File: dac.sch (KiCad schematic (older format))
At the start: 1 part, among them U701 DAC8568C

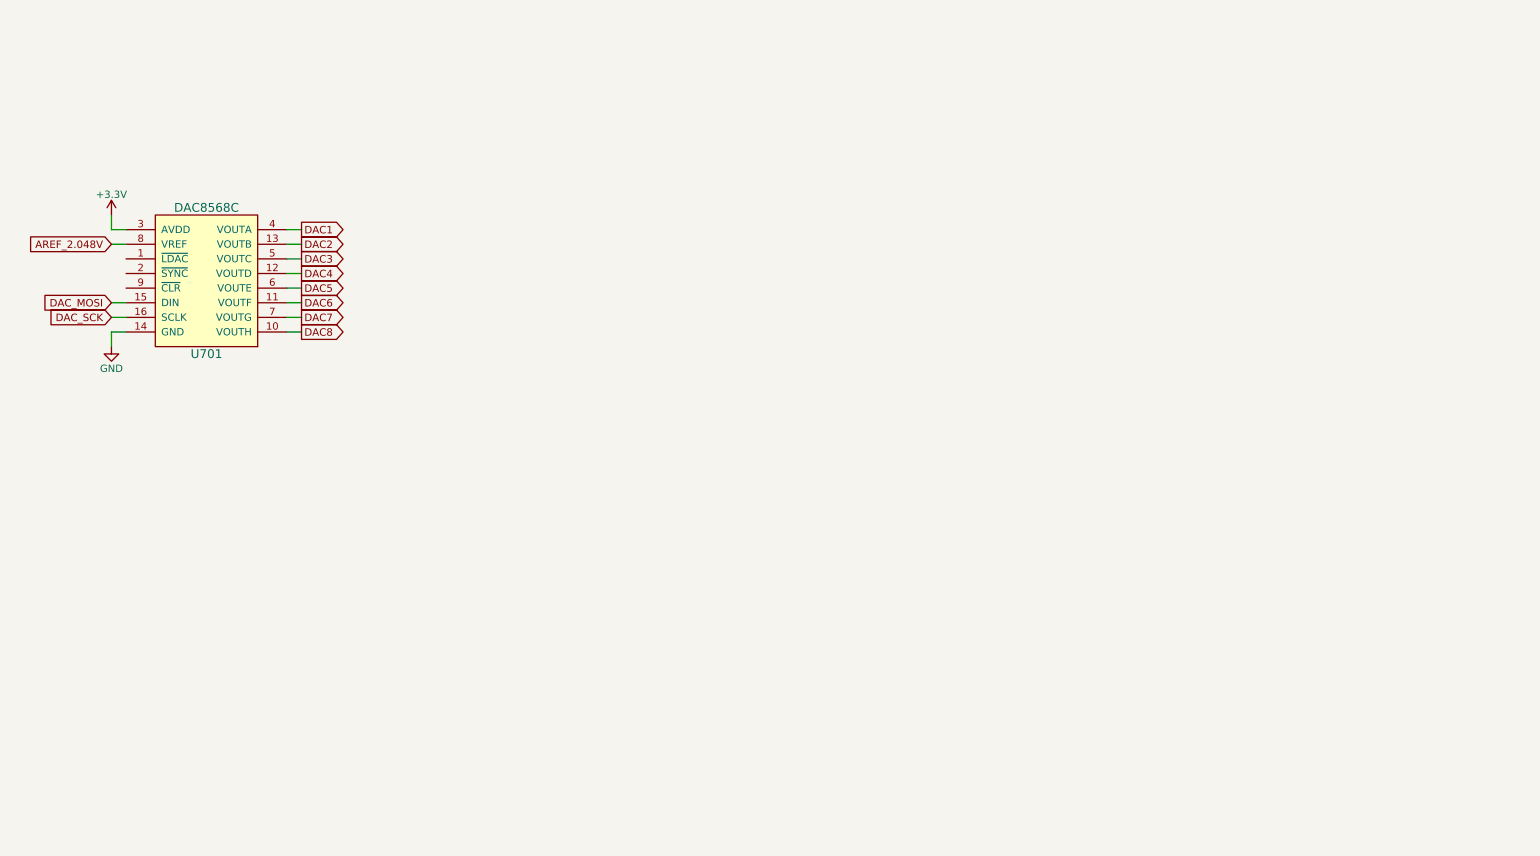
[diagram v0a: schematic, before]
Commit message: work in progress
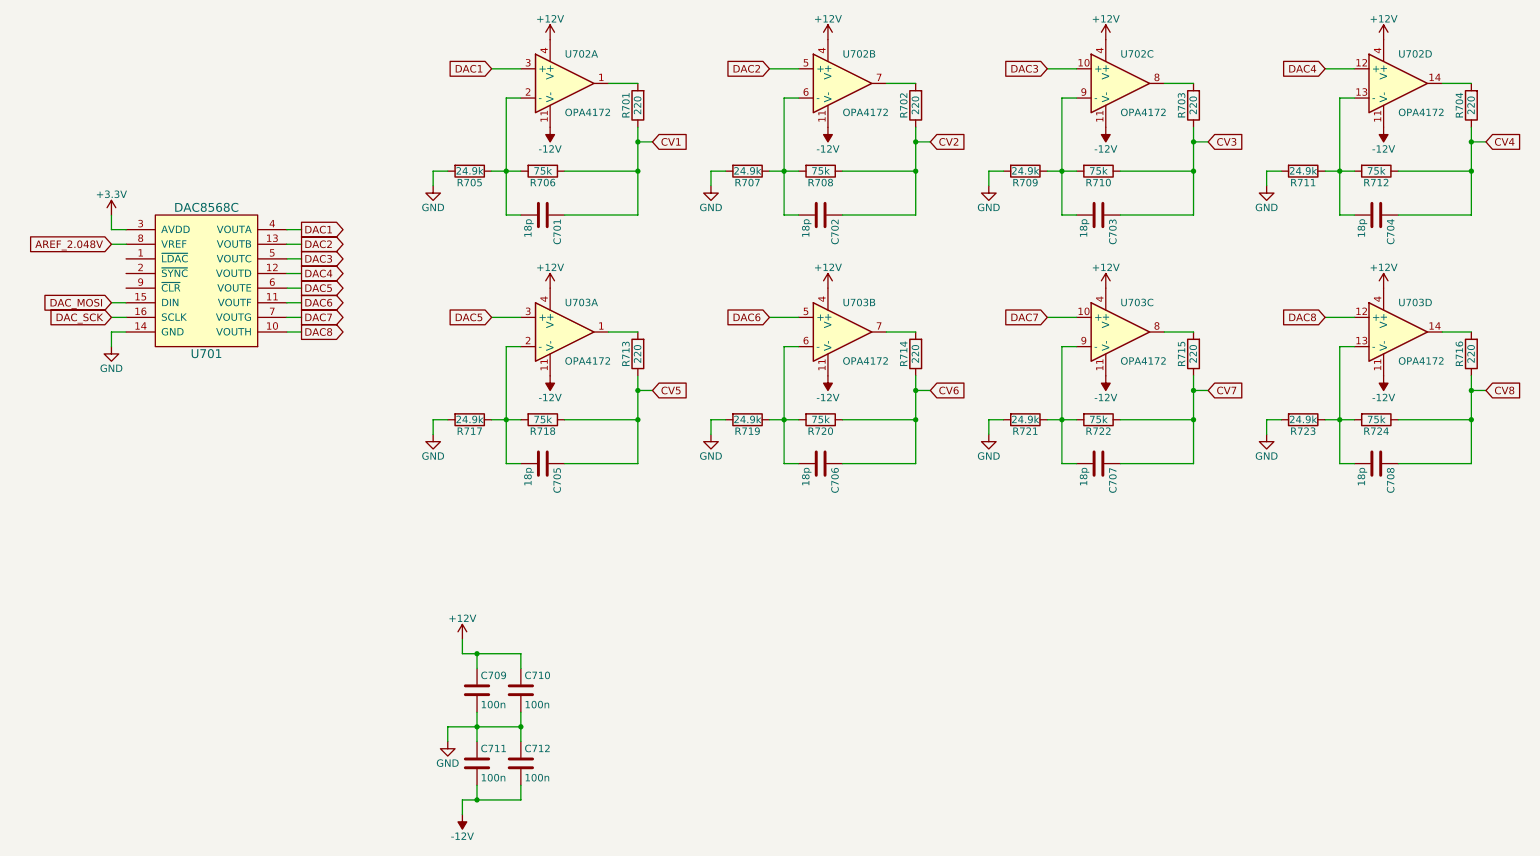
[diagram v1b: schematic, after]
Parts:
- added C701, C702, C703, C704, C705, C706, C707, C708: 18p, Capacitors_SMD:C_0603, symbol C
- added C709, C710, C711, C712: 100n, Capacitors_SMD:C_0603, symbol C
- added R701, R702, R703, R704, R713, R714, R715, R716: 220, Resistors_SMD:R_0603, symbol R
- added R705, R707, R709, R711, R717, R719, R721, R723: 24.9k, Resistors_SMD:R_0603, symbol R
- added R706, R708, R710, R712, R718, R720, R722, R724: 75k, Resistors_SMD:R_0603, symbol R
- added U702, U703: OPA4172, Housings_SOIC:SOIC-14_3.9x8.7mm_Pitch1.27mm, symbol OPA4134
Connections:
- net DAC1: now also U702.3 (+)
- net DAC2: now also U702.5 (+)
- net DAC3: now also U702.10 (+)
- net DAC4: now also U702.12 (+)
- net DAC5: now also U703.3 (+)
- net DAC6: now also U703.5 (+)
- net DAC7: now also U703.10 (+)
- net DAC8: now also U703.12 (+)
- net GND: now also C709.2, C710.2, C711.1, C712.1, R705.2, R707.2, R709.2, R711.2, R717.2, R719.2, R721.2, R723.2
- new net: C702.2, R707.1, R708.2, U702.6 (-)
- new net: R702.2, U702.7
- new net: C704.2, R711.1, R712.2, U702.13 (-)
- new net: R704.2, U702.14
- new net: C706.2, R719.1, R720.2, U703.6 (-)
- new net: R714.2, U703.7
- new net: R701.2, U702.1
- new net: C701.2, R705.1, R706.2, U702.2 (-)
- new net: R703.2, U702.8
- new net: C703.2, R709.1, R710.2, U702.9 (-)
- new net: R713.2, U703.1
- new net: C705.2, R717.1, R718.2, U703.2 (-)
- new net: R715.2, U703.8
- new net: C707.2, R721.1, R722.2, U703.9 (-)
- new net: C708.2, R723.1, R724.2, U703.13 (-)
- new net: R716.2, U703.14
- new net +12V: C709.1, C710.1, U702.4 (V+), U702.4 (V+), U702.4 (V+), U702.4 (V+), U703.4 (V+), U703.4 (V+), U703.4 (V+), U703.4 (V+)
- new net -12V: C711.2, C712.2, U702.11 (V-), U702.11 (V-), U702.11 (V-), U702.11 (V-), U703.11 (V-), U703.11 (V-), U703.11 (V-), U703.11 (V-)
- new net CV1: C701.1, R701.1, R706.1
- new net CV2: C702.1, R702.1, R708.1
- new net CV3: C703.1, R703.1, R710.1
- new net CV4: C704.1, R704.1, R712.1
- new net CV5: C705.1, R713.1, R718.1
- new net CV6: C706.1, R714.1, R720.1
- new net CV7: C707.1, R715.1, R722.1
- new net CV8: C708.1, R716.1, R724.1

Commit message: more work
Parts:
- C701, C702, C703, C704, C705, C706, C707, C708: MFN (none) -> Murata; MFP (none) -> GRM1885C1H180JA01J
- C709, C710, C711, C712: MFN (none) -> Murata; MFP (none) -> GRM188R71E104JA01J
- U702, U703: MFN (none) -> Texas Instruments; MFP (none) -> OPA4172IPW

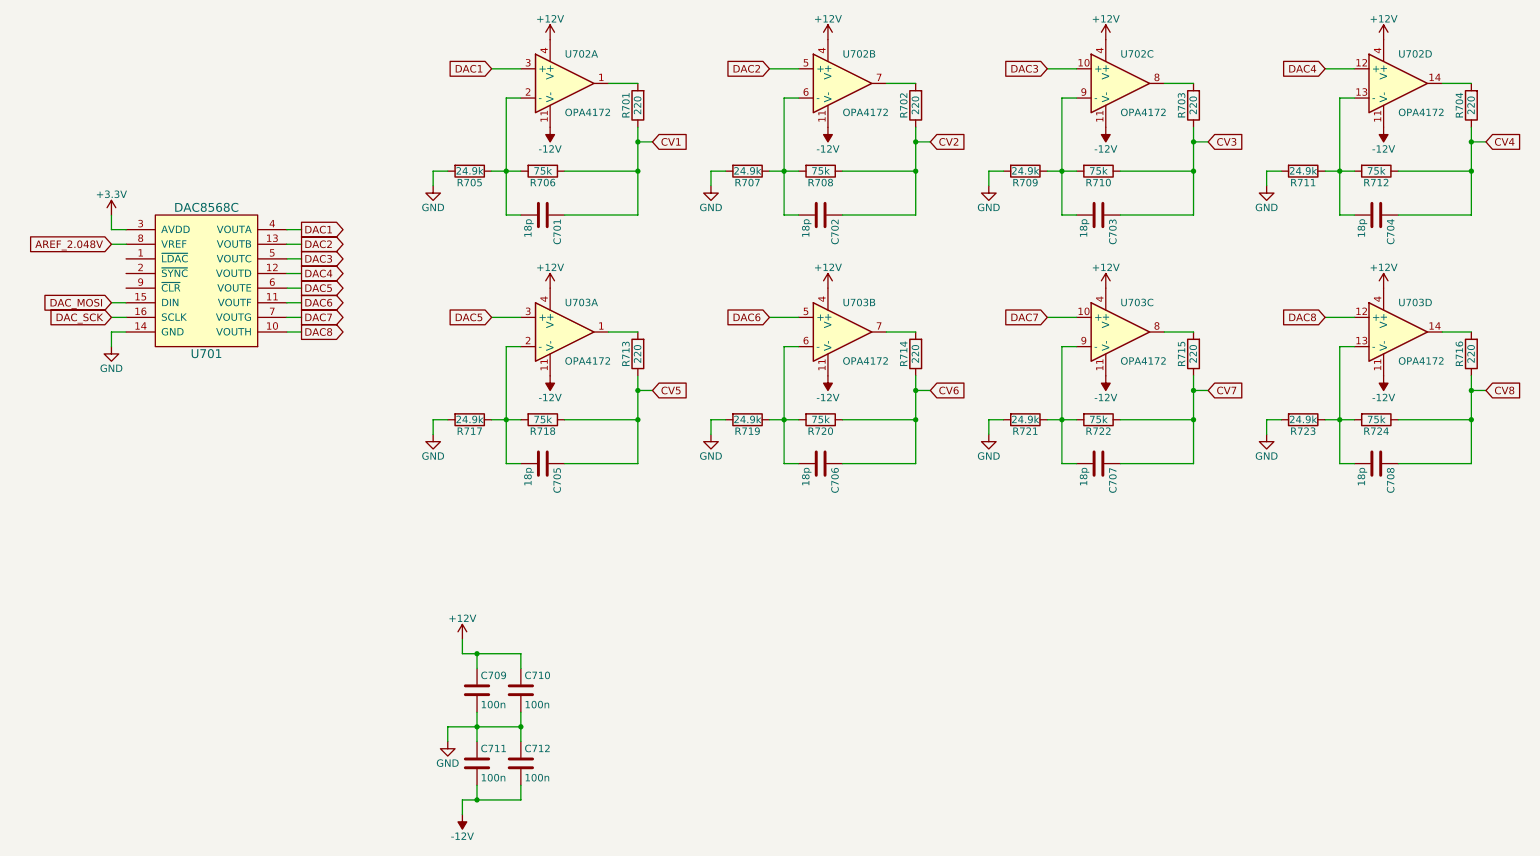
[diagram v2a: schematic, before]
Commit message: more work on layout
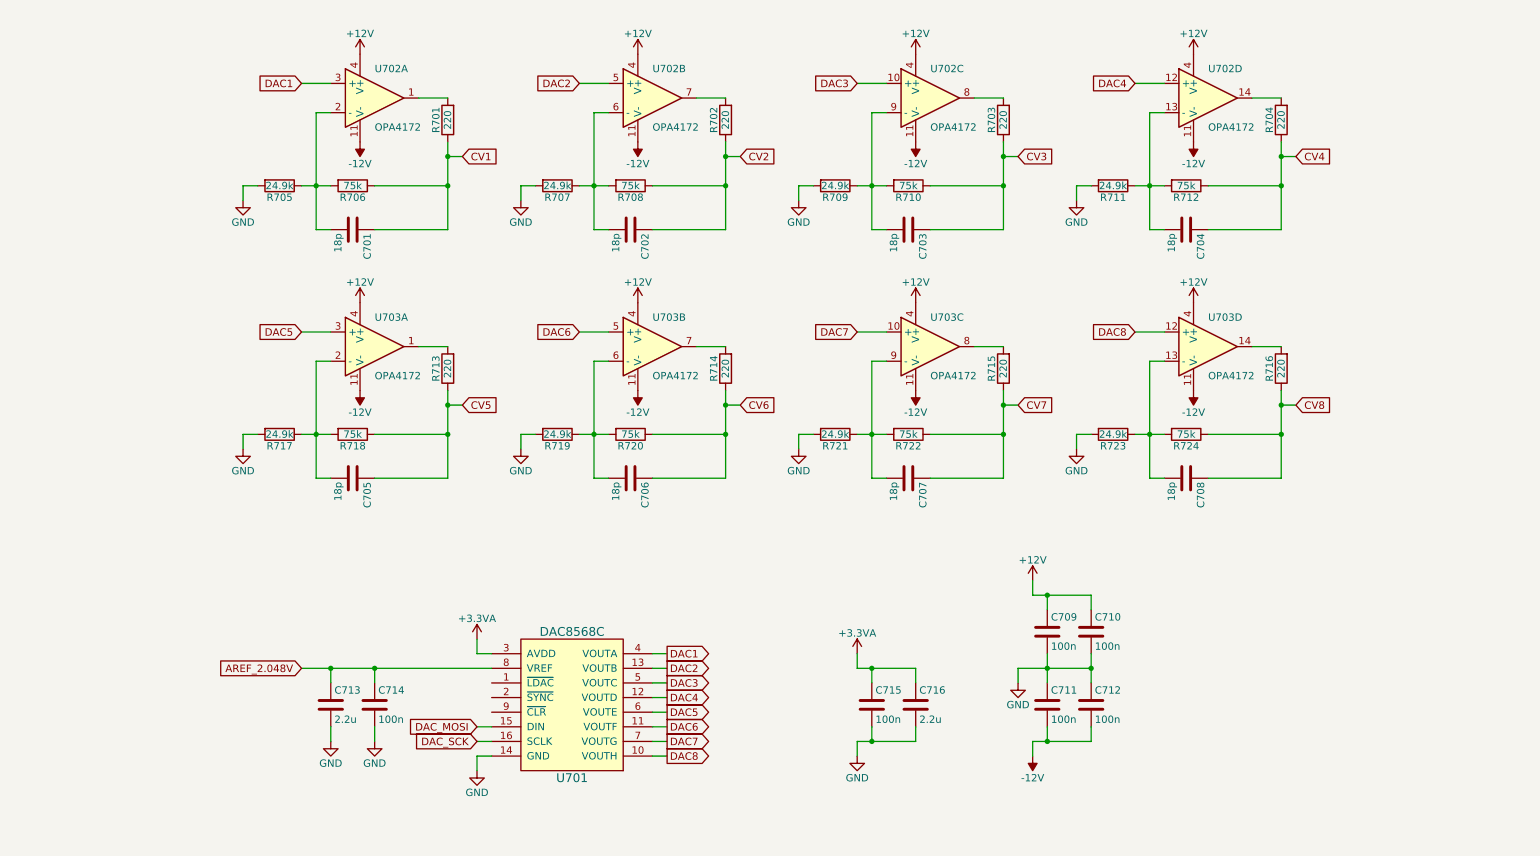
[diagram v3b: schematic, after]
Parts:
- added C713, C716: 2.2u, Capacitors_SMD:C_0805, symbol C
- added C714, C715: 100n, Capacitors_SMD:C_0603, symbol C
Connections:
- net AREF_2.048V: now also C713.1, C714.1
- net GND: now also C713.2, C714.2, C715.2, C716.2
- net +3V3 renamed +3.3VA
- net +3.3VA: now also C715.1, C716.1
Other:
- moved on the sheet: C701, C702, C703, C704, C705, C706, C707, C708, C709, C710, C711, C712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

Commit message: redesign in progress
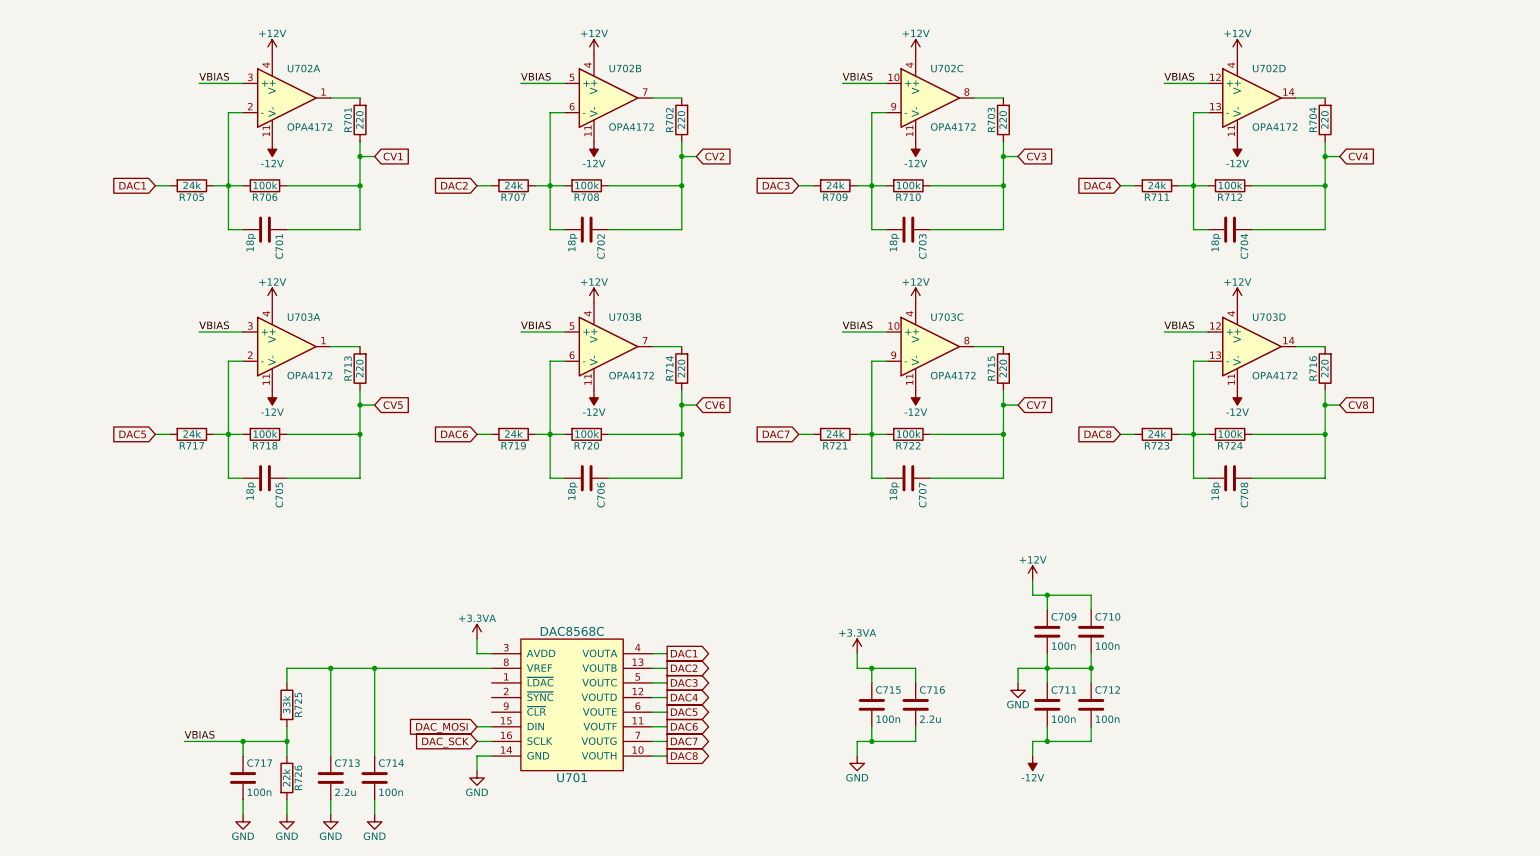
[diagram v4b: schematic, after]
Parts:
- added C717: 100n, Capacitors_SMD:C_0603, symbol C
- added R725: 33k, Resistors_SMD:R_0603, symbol R
- added R726: 22k, Resistors_SMD:R_0603, symbol R
- R705, R707, R709, R711, R717, R719, R721, R723: value 24.9k -> 24k; MFP ERJ-3EKF2492V -> ERJ-3EKF2402V
- R706, R708, R710, R712, R718, R720, R722, R724: value 75k -> 100k; MFP ERJ-3EKF7502V -> ERJ-3EKF1003V
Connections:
- net DAC1: now also R705.2; no longer U702.3 (+)
- net DAC2: now also R707.2; no longer U702.5 (+)
- net DAC3: now also R709.2; no longer U702.10 (+)
- net DAC4: now also R711.2; no longer U702.12 (+)
- net DAC5: now also R717.2; no longer U703.3 (+)
- net DAC6: now also R719.2; no longer U703.5 (+)
- net DAC7: now also R721.2; no longer U703.10 (+)
- net DAC8: now also R723.2; no longer U703.12 (+)
- net GND: now also C717.2, R726.2; no longer R705.2, R707.2, R709.2, R711.2, R717.2, R719.2, R721.2, R723.2
- net AREF_2.048V: no longer names the net of C713.1, C714.1, U701.8 (VREF)
- net AREF_2.048V: now also R725.1
- new net VBIAS: C717.1, R725.2, R726.1, U702.10 (+), U702.12 (+), U702.3 (+), U702.5 (+), U703.10 (+), U703.12 (+), U703.3 (+), U703.5 (+)
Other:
- moved on the sheet: C701, C702, C704, C705, C706, C708, C713, C714, R701, R702, R704, R705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
